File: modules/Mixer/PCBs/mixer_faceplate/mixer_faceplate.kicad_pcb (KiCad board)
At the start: 2 copper layers, 40.3 x 128.5 mm, 0 parts

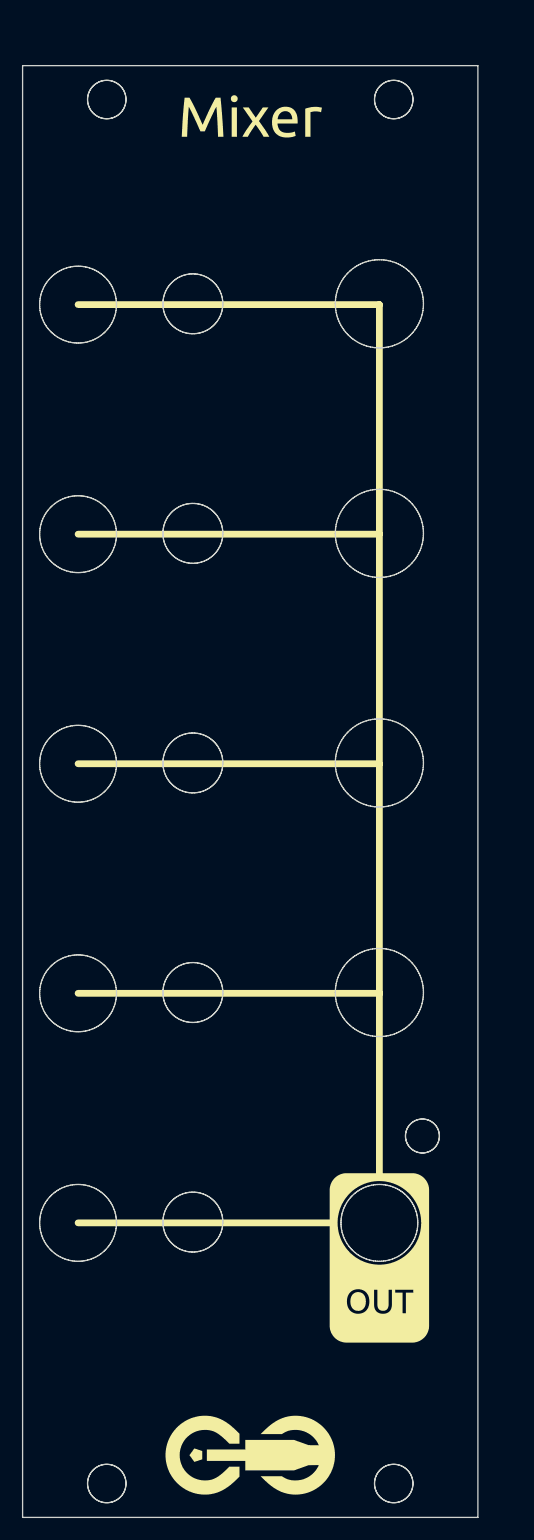
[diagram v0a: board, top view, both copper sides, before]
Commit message: adjust mixer PCB
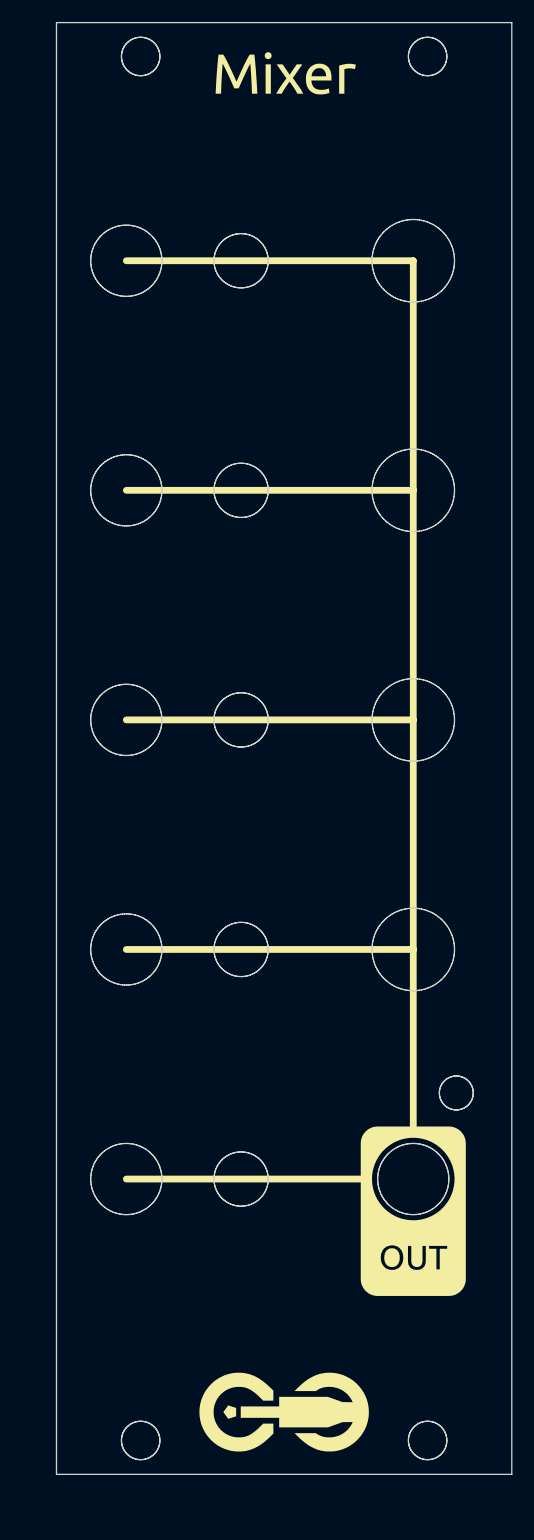
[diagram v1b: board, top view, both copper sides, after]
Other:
- outline, holes or cut-outs redrawn
